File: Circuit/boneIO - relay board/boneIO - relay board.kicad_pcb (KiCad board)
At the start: 2 copper layers, 197 x 102 mm, 68 parts, among them J1 Screw_Terminal_01x04, J10 Screw_Terminal_01x04, J11 Screw_Terminal_01x04, J12 Screw_Terminal_01x04, J13 Screw_Terminal_01x04, J14 Conn_02x04_Odd_Even, J2 Screw_Terminal_01x04, J4 Screw_Terminal_01x04, J5 Screw_Terminal_01x04, J6 Screw_Terminal_01x04, J7 Screw_Terminal_01x04, J8 Screw_Terminal_01x04, J9 Screw_Terminal_01x04, K1 RM85-2011-35-1005, K10 RM85-2011-35-1005, K11 RM85-2011-35-1005, K12 RM85-2011-35-1005, K13 RM85-2011-35-1005, K14 RM85-2011-35-1005, K15 RM85-2011-35-1005, K16 RM85-2011-35-1005, K17 RM85-2011-35-1005, K18 RM85-2011-35-1005, K19 RM85-2011-35-1005, K2 RM85-2011-35-1005, K20 RM85-2011-35-1005, K21 RM85-2011-35-1005, K22 RM85-2011-35-1005, K23 RM85-2011-35-1005, K24 RM85-2011-35-1005, K3 RM85-2011-35-1005, K4 RM85-2011-35-1005, K5 RM85-2011-35-1005, K6 RM85-2011-35-1005, K7 RM85-2011-35-1005, K8 RM85-2011-35-1005, K9 RM85-2011-35-1005, SW1 SW_DIP_x03, SW2 SW_DIP_x03, SW3 SW_DIP_x03, U1 MCP9808_MSOP, U2 MCP23017_SS, U3 MCP23017_SS, U4 ULN2803A, U5 ULN2803A, U6 ULN2803A

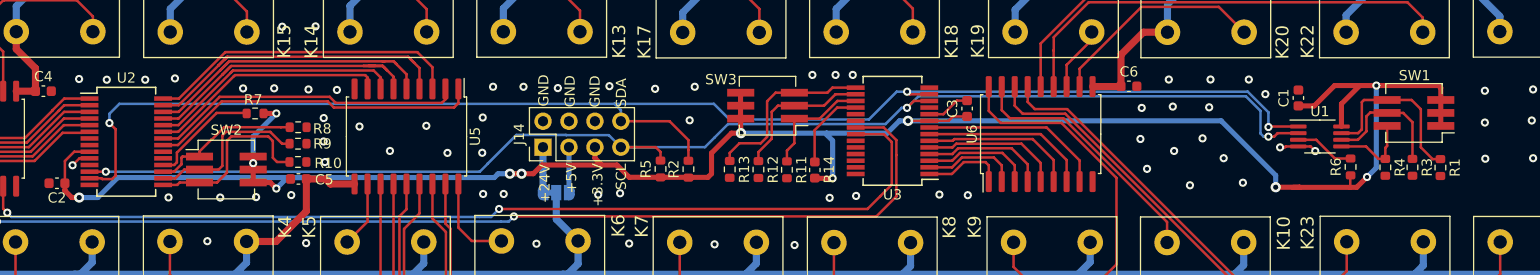
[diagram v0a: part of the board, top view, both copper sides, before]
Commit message: 05.11.2021
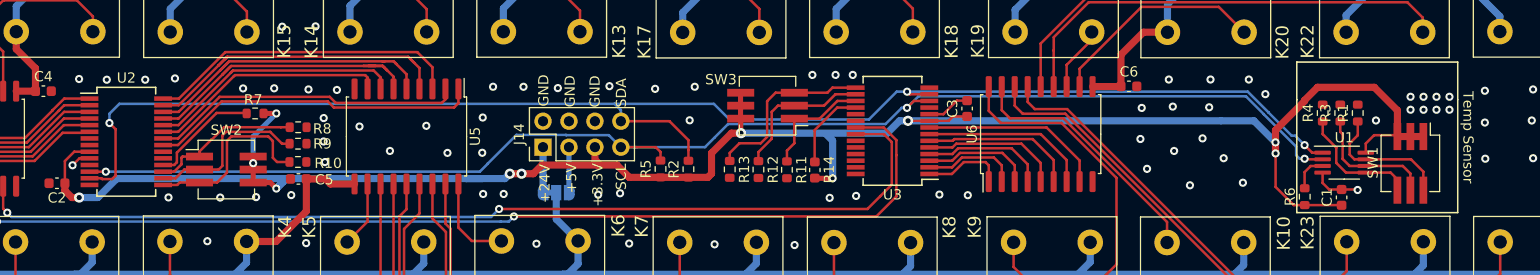
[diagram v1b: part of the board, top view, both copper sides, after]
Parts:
- moved C1 10.6 mm to (456.3, 320.6)
- moved R1 9.69 mm to (457.9, 312.4), turned to 90 degrees
- moved R3 8.84 mm to (456.2, 312.4), turned to 90 degrees
- moved R4 8.11 mm to (454.4, 312.4), turned to 90 degrees
- moved R6 5.35 mm to (452.7, 320.6)
- moved SW1 4.95 mm to (463.0, 317.3), turned to 270 degrees
- moved U1 3.50 mm to (456.5, 317.2)
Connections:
- SW1 pad 4: Net-(R1-Pad1) -> Net-(R4-Pad1)
- SW1 pad 6: Net-(R4-Pad1) -> Net-(R1-Pad1)
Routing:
- net +3V3: track 212.2 -> 273.7 mm, vias 12 -> 11
- net Net-(R1-Pad1): track 17.2 -> 13.3 mm
- net Net-(R4-Pad1): track 8.10 -> 11.9 mm
- net SDA: track 143.6 -> 146.2 mm
- net SCL: track 133.1 -> 135.5 mm
- net Net-(R6-Pad2): track 5.88 -> 3.66 mm
- net GND: track 9.85 -> 10.9 mm, vias 101 -> 109
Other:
- board text added: "Temp Sensor"
